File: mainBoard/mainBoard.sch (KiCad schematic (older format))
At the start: 60 parts, among them J1 program, J2 uniwersal-board2, SW1 reset, U1 STM32F407VGTx, U2 SMF05C / MMQA5V6T3G, U3 usb-micro, U4 MIC5504-3.3YM5, Y1 32kHz, Y2 8/16MHz

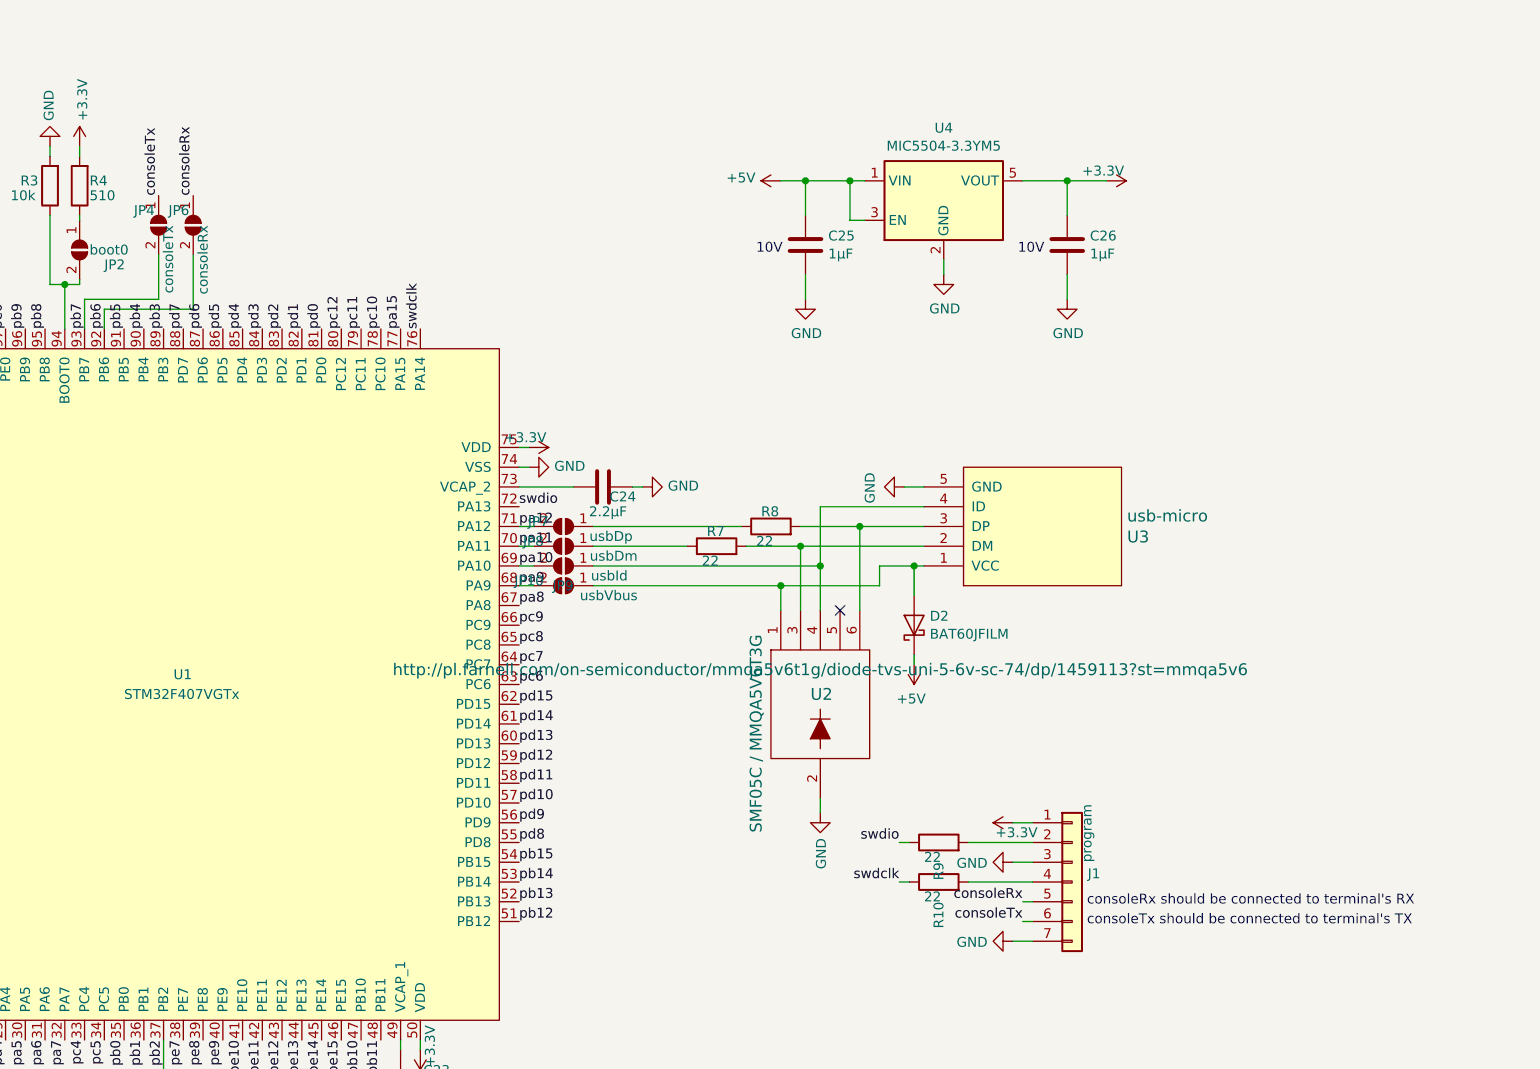
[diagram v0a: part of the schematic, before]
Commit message: Bug-fixes. 3 battery soldered and working.
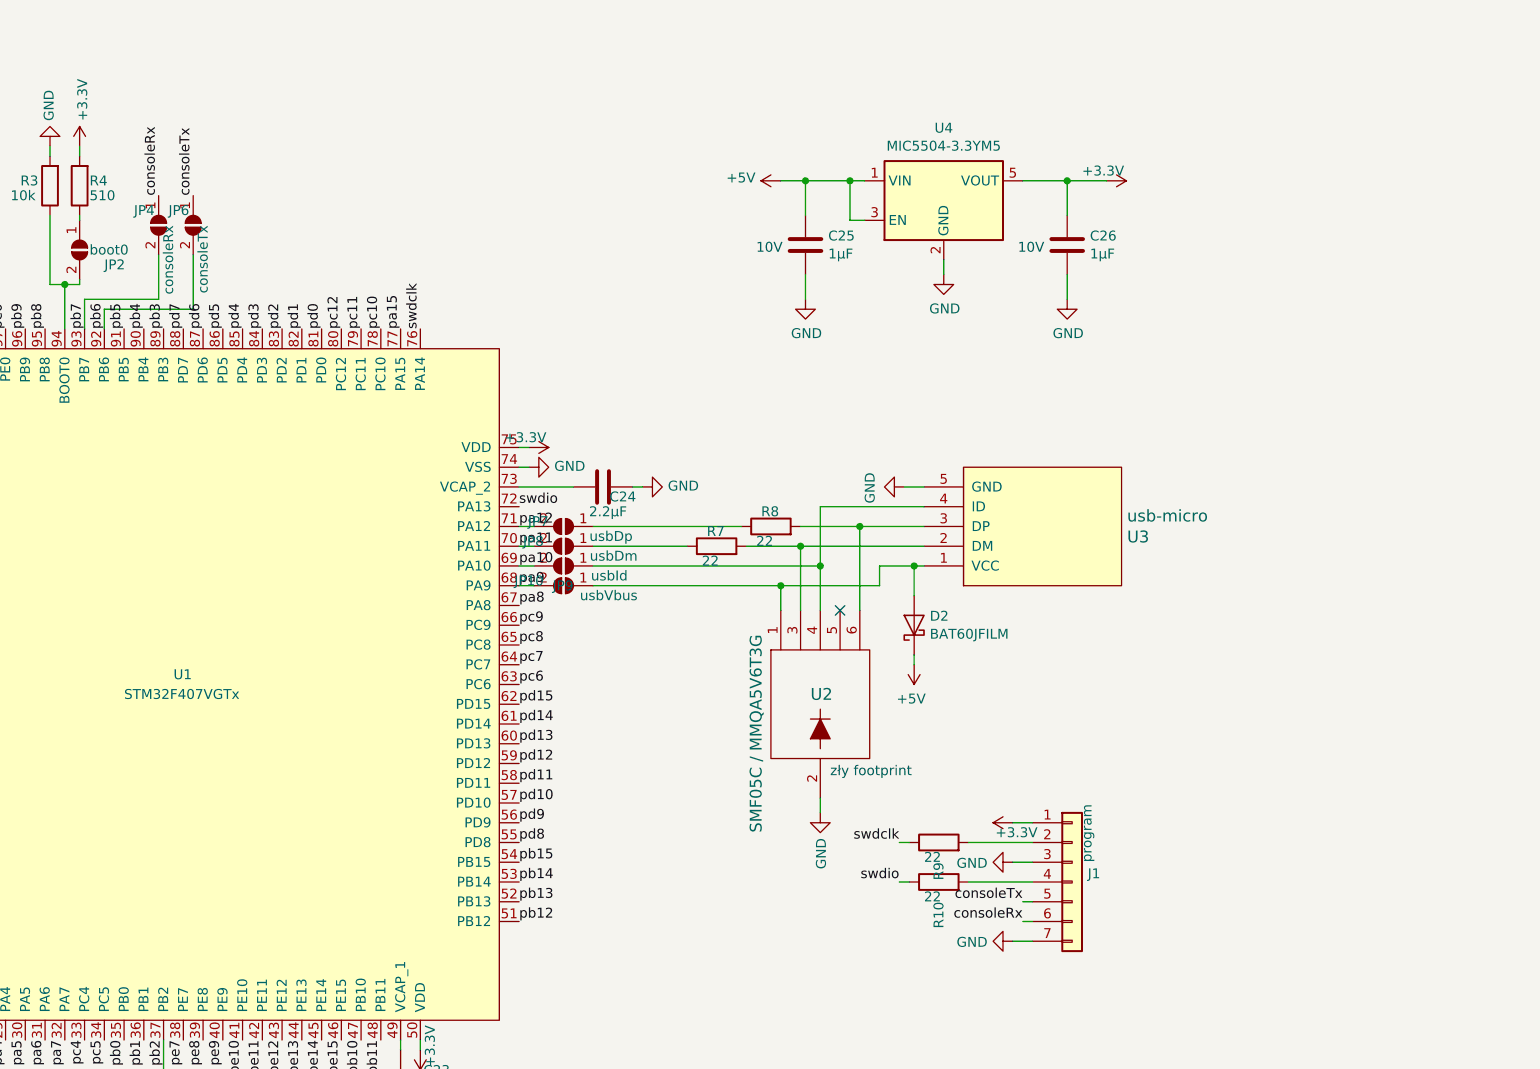
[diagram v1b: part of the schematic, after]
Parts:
- JP4: value consoleTx -> consoleRx
- JP6: value consoleRx -> consoleTx
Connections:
- net consoleRx: now also J1.6 (Pin_6), JP4.1 (A); no longer J1.5 (Pin_5), JP6.1 (A)
- net consoleTx: now also J1.5 (Pin_5), JP6.1 (A); no longer J1.6 (Pin_6), JP4.1 (A)
- net swdclk: now also R9.1; no longer R10.1
- net swdio: now also R10.1; no longer R9.1
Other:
- note added: "zły footprint"
- note removed: "consoleRx should be connected to terminal's RX"
- note removed: "consoleTx should be connected to terminal's TX"
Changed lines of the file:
@@
 Wire Wire Line
 	10425 5250 10525 5250
+Text Label 9850 4950 2    50   ~ 0
+swdio
 Text Label 9850 4750 2    50   ~ 0
-swdio
-Text Label 9850 4950 2    50   ~ 0
 swdclk
+Text Label 10475 5150 2    50   ~ 0
+consoleRx
 Text Label 10475 5050 2    50   ~ 0
-consoleRx
-Text Label 10475 5150 2    50   ~ 0
 consoleTx
 Text Label 7925 3050 0    50   ~ 0
@@
 swdclk
 Text Label 6100 1475 1    50   ~ 0
-consoleTx
-Text Notes 10800 5075 0    50   ~ 0
-consoleRx should be connected to terminal's RX
-Text Notes 10800 5175 0    50   ~ 0
-consoleTx should be connected to terminal's TX
+consoleRx
 $Comp
 L iwasz-kicad:SMF05C U2
@@
 F 1 "SMF05C / MMQA5V6T3G" V 9125 3050 60  0000 L CNN
 F 2 "Package_TO_SOT_SMD:SOT-363_SC-70-6" H 9450 3875 60  0001 C CNN
-F 3 "http://pl.farnell.com/on-semiconductor/mmqa5v6t1g/diode-tvs-uni-5-6v-sc-74/dp/1459113?st=mmqa5v6" H 9450 3875 60  0000 C CNN
+F 3 "http://pl.farnell.com/on-semiconductor/mmqa5v6t1g/diode-tvs-uni-5-6v-sc-74/dp/1459113?st=mmqa5v6" H 9450 3875 60  0001 C CNN
 	1    9450 3875
 	1    0    0    -1
@@
 P 6100 1625
 F 0 "JP4" V 6025 1500 50  0000 L CNN
-F 1 "consoleTx" H 6100 1675 50  0000 L CNN
+F 1 "consoleRx" H 6100 1675 50  0000 L CNN
 F 2 "Jumper:SolderJumper-2_P1.3mm_Bridged_RoundedPad1.0x1.5mm" H 6100 1625 50  0001 C CNN
 F 3 "~" H 6100 1625 50  0001 C CNN
@@
 	6100 2000 6100 1775
 Text Label 6275 1475 1    50   ~ 0
-consoleRx
+consoleTx
 $Comp
 L Jumper:SolderJumper_2_Open JP6
@@
 P 6275 1625
 F 0 "JP6" V 6200 1500 50  0000 L CNN
-F 1 "consoleRx" H 6275 1675 50  0000 L CNN
+F 1 "consoleTx" H 6275 1675 50  0000 L CNN
 F 2 "Jumper:SolderJumper-2_P1.3mm_Bridged_RoundedPad1.0x1.5mm" H 6275 1625 50  0001 C CNN
 F 3 "~" H 6275 1625 50  0001 C CNN
@@
 Wire Wire Line
 	1200 5475 1250 5475
+Text Notes 9500 4425 0    50   ~ 0
+zły footprint
 $EndSCHEMATC
